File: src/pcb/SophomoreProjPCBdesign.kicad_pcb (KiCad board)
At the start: 2 copper layers, 90.3 x 46.8 mm, 20 parts, among them J1 AudioJack2, J2 AudioJack2, J3 Power_Conn_01x02, Q1 NJFET, SW2 SW_SPST, U1 LM386

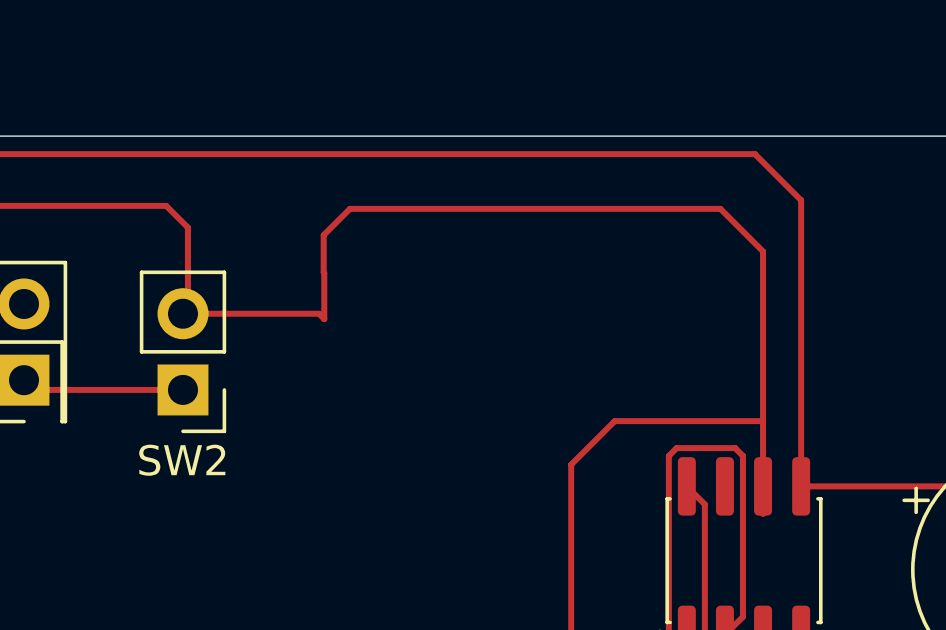
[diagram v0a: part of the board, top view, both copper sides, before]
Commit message: pcb: fixed messay trace
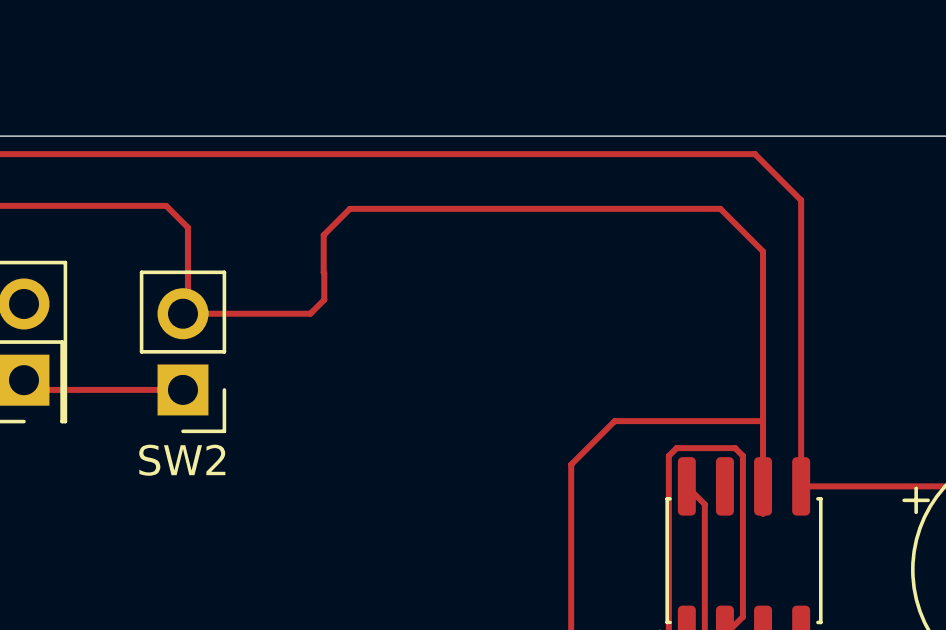
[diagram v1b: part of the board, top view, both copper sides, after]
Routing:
- net Net-(Q1-D): track 126.4 -> 125.9 mm
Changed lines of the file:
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@@
 	)
 	(segment
-		(start 150.6 69.225)
-		(end 150.6 70.475)
-		(width 0.2)
-		(layer "F.Cu")
-		(net "Net-(Q1-D)")
-	)
-	(segment
-		(start 151.475 68.35)
-		(end 150.6 69.225)
+		(start 163.825 68.35)
+		(end 165.245 69.77)
 		(width 0.2)
 		(layer "F.Cu")
@@
 	)
 	(segment
+		(start 165.245 69.77)
+		(end 165.245 75.425)
+		(width 0.2)
+		(layer "F.Cu")
+		(net "Net-(Q1-D)")
+	)
+	(segment
 		(start 158.85 76.875)
 		(end 160.3 75.425)
@@
 	)
 	(segment
+		(start 145.91 71.845)
+		(end 150.155 71.845)
+		(width 0.2)
+		(layer "F.Cu")
+		(net "Net-(Q1-D)")
+	)
+	(segment
 		(start 146.075 71.68)
 		(end 146.075 68.975)
@@
 	)
 	(segment
+		(start 150.62 71.38)
+		(end 150.62 70.495)
+		(width 0.2)
+		(layer "F.Cu")
+		(net "Net-(Q1-D)")
+	)
+	(segment
 		(start 145.91 71.845)
 		(end 146.075 71.68)
@@
 	)
 	(segment
-		(start 163.825 68.35)
-		(end 151.475 68.35)
-		(width 0.2)
-		(layer "F.Cu")
-		(net "Net-(Q1-D)")
-	)
-	(segment
 		(start 145.35 68.25)
 		(end 133 68.25)
@@
 	)
 	(segment
-		(start 165.245 69.77)
-		(end 163.825 68.35)
-		(width 0.2)
-		(layer "F.Cu")
-		(net "Net-(Q1-D)")
-	)
-	(segment
 		(start 113.625 81.425)
 		(end 113.625 71.3)
@@
 	)
 	(segment
-		(start 150.44 71.845)
-		(end 150.62 72.025)
-		(width 0.2)
-		(layer "F.Cu")
-		(net "Net-(Q1-D)")
-	)
-	(segment
 		(start 113.625 71.3)
 		(end 114.96 69.965)
@@
 	)
 	(segment
-		(start 145.91 71.845)
-		(end 150.44 71.845)
-		(width 0.2)
-		(layer "F.Cu")
-		(net "Net-(Q1-D)")
-	)
-	(segment
-		(start 150.62 70.495)
-		(end 150.62 72.025)
-		(width 0.2)
-		(layer "F.Cu")
-		(net "Net-(Q1-D)")
-	)
-	(segment
 		(start 158.015 90.86)
 		(end 158.85 90.025)
@@
 	)
 	(segment
+		(start 150.62 70.495)
+		(end 150.6 70.475)
+		(width 0.2)
+		(layer "F.Cu")
+		(net "Net-(Q1-D)")
+	)
+	(segment
 		(start 131.85 69.4)
 		(end 131.85 83.8)
@@
 	)
 	(segment
+		(start 150.6 69.225)
+		(end 151.475 68.35)
+		(width 0.2)
+		(layer "F.Cu")
+		(net "Net-(Q1-D)")
+	)
+	(segment
 		(start 133 68.25)
 		(end 131.85 69.4)
@@
 	)
 	(segment
+		(start 150.155 71.845)
+		(end 150.62 71.38)
+		(width 0.2)
+		(layer "F.Cu")
+		(net "Net-(Q1-D)")
+	)
+	(segment
 		(start 131.69 90.21)
 		(end 131.69 84.165)
@@
 	)
 	(segment
+		(start 150.6 70.475)
+		(end 150.6 69.225)
+		(width 0.2)
+		(layer "F.Cu")
+		(net "Net-(Q1-D)")
+	)
+	(segment
 		(start 165.245 77.6)
 		(end 165.245 75.425)
@@
 	)
 	(segment
-		(start 165.245 75.425)
-		(end 165.245 69.77)
-		(width 0.2)
-		(layer "F.Cu")
-		(net "Net-(Q1-D)")
-	)
-	(segment
-		(start 150.6 70.475)
-		(end 150.62 70.495)
-		(width 0.2)
-		(layer "F.Cu")
+		(start 151.475 68.35)
+		(end 163.825 68.35)
+		(width 0.2)
+		(layer "F.Cu")
